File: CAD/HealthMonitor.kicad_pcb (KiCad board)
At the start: 2 copper layers, 70 x 30 mm, 114 parts, among them J1 BAT_T, J10 SDA, J11 SCL, J12 DIS_SW, J13 BAT_CHRG, J14 USBDP, J15 USBDM, J16 USB_V, J17 VBUS, J18 D+, J19 D-, J2 TEG+, J20 SDA, J21 SCL, J22 VCC, J23 GND, J24 BAT_CHRG, J25 DIS_SW, J3 TEG-, J4 BAT-, J5 BAT+, J6 USB_C_Receptacle_USB2.0, J7 Conn_02x05_Odd_Even, J8 VCC, J9 GND, U1 MAX17048G+T10, U10 AT24CS02-XHM, U11 BT832L, U12 CP2102N-A01-GQFN24, U13 ADG884BRMZ, U2 ADP5092ACPZ-1-R7, U3 LTC4079IDD-PBF, U4 LD39015M33R, U5 BH1792GLC, U6 LSM6DS33TR, U7 TXB0104RUT, U8 MAX1921EUT18+, U9 MAX86141ENP+, Y1 ABS06-32.768KHZ-T

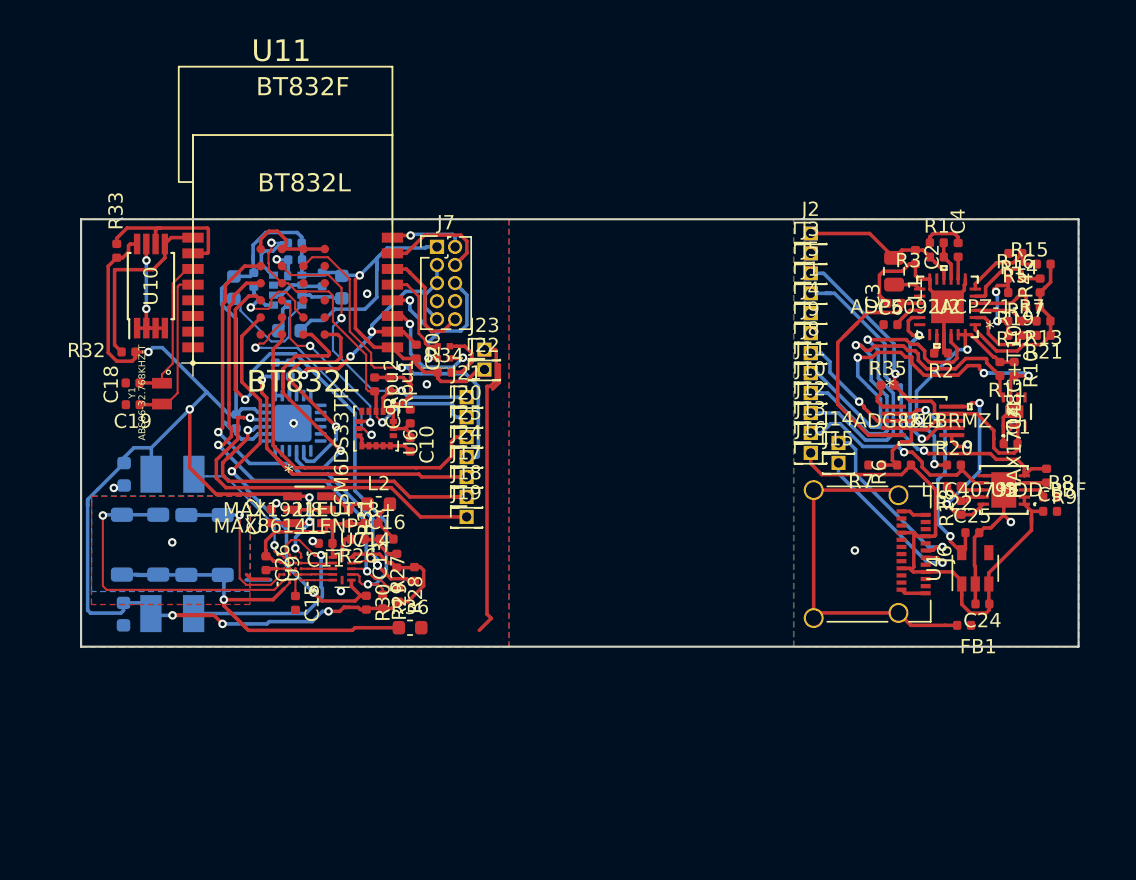
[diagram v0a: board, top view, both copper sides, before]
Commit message: rescue commit
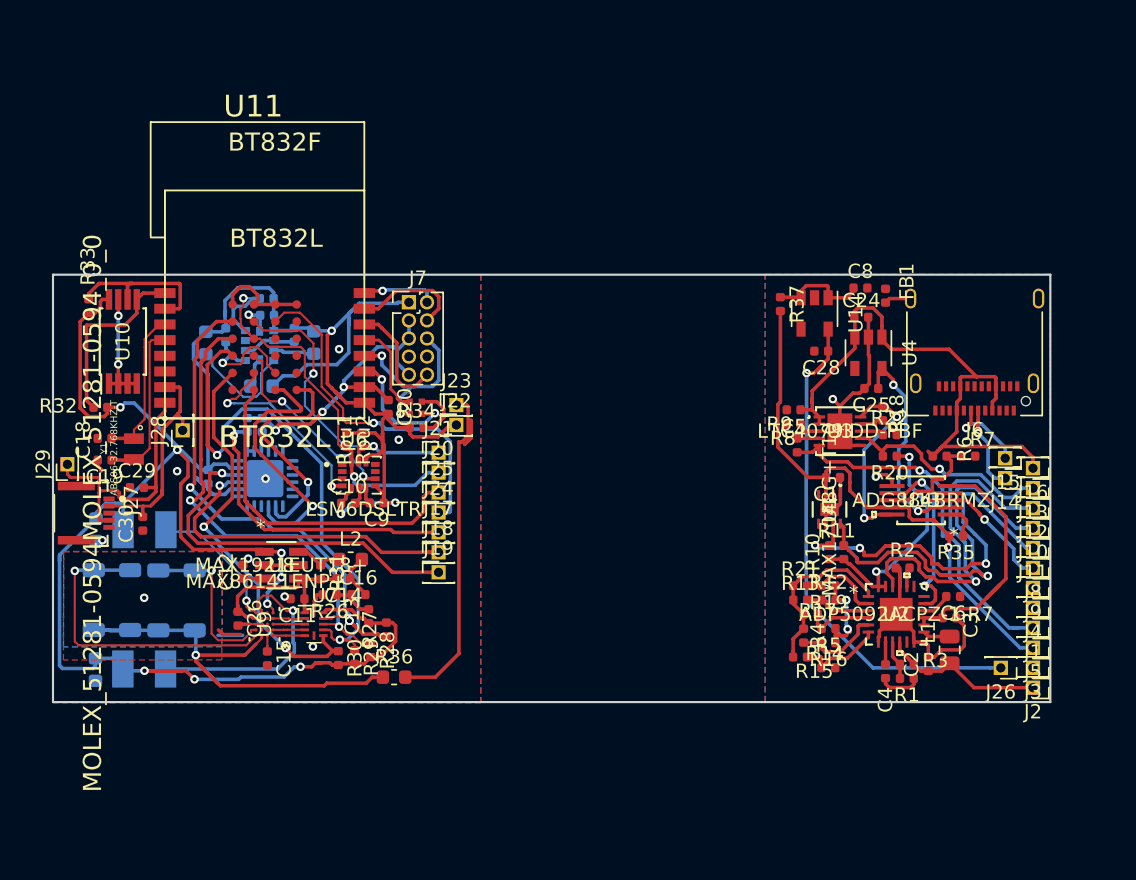
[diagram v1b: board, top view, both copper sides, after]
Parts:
- added C28: 1u, Capacitor_SMD:C_0402_1005Metric, F.Cu at (153.9, 105.4)
- added C29: 12p, Capacitor_SMD:C_0402_1005Metric, F.Cu at (105.9, 114.9)
- added C30: 12p, Capacitor_SMD:C_0402_1005Metric, F.Cu at (106.3, 117.5)
- added C8: 1u, Capacitor_SMD:C_0402_1005Metric, F.Cu at (156.7, 100.9)
- added J26: Conn_01x01_Male, Connector_PinHeader_1.27mm:PinHeader_1x01_P1.27mm_Vertical, F.Cu at (166.5, 127.6)
- added J27: MOLEX_51281-0594MOLEX_51281-0594_0_0, Molex - 51281-0594:Molex - 51281-0594-MOLEX_51281-0594_0, F.Cu at (102.8, 116.7)
- added J28: Conn_01x01_Male, Connector_PinHeader_1.27mm:PinHeader_1x01_P1.27mm_Vertical, F.Cu at (109.1, 110.9)
- added J29: Conn_01x01_Male, Connector_PinHeader_1.27mm:PinHeader_1x01_P1.27mm_Vertical, F.Cu at (101.0, 113.3)
- added R37: 0, Resistor_SMD:R_0402_1005Metric, F.Cu at (151.1, 102.1)
- added U14: LD39015M33R, Package_TO_SOT_SMD:SOT-23-5, F.Cu at (153.4, 102.7)
- C10: value 10µF -> 100nF
- C11, C13: value 0.1µF -> 0.1u
- J6: footprint footprints:USB_C_Receptacle_Amphenol_12401610E4-2A_CircularHoles -> Connector_USB:USB_C_Receptacle_Amphenol_12401610E4-2A
- U6: value LSM6DS33TR -> LSM6DSLTR; footprint LSM6DS33TR:PQFN50P300X300X86-16N -> LSM6DSLTR:PQFN50P300X250X86-14N
- moved J2 35.5 mm to (168.8, 129.0), turned to 180 degrees
- moved J3 33.0 mm to (168.8, 127.6), turned to 180 degrees
- moved R15 32.4 mm to (152.4, 126.8), turned to 0 degrees
- moved R14 31.9 mm to (154.4, 127.6), turned to 180 degrees
- moved R1 30.6 mm to (159.9, 128.3), turned to 180 degrees
- moved J5 30.6 mm to (168.8, 126.2), turned to 180 degrees
- moved C4 30.0 mm to (158.4, 127.8), turned to 270 degrees
- moved R17 29.7 mm to (152.7, 125.3), turned to 270 degrees
- moved R16 28.7 mm to (154.4, 125.8), turned to 180 degrees
- moved R3 28.7 mm to (159.9, 127.3), turned to 0 degrees
- moved C2 28.6 mm to (161.4, 127.3), turned to 90 degrees
- moved J1 28.2 mm to (168.8, 124.8), turned to 180 degrees
- moved R5 27.0 mm to (154.4, 124.8), turned to 180 degrees
- moved L1 26.9 mm to (162.9, 126.3), turned to 270 degrees
- moved R4 26.6 mm to (153.2, 123.8), turned to 180 degrees
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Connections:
- Rpu1 pad 1: +3V3 -> /SCL
- Rpu1 pad 2: /SCL -> +3V3
- U6 pad 1: +3V3 -> GND
- U6 pad 10: GND -> (no net)
- U6 pad 11: GND -> (no net)
- U6 pad 12: GND -> +3V3
- U6 pad 13: GND -> /SCL
- U6 pad 14: Net-(U6-Pad14) -> /SDA
- U6 pad 2: /SCL -> Net-(U6-Pad2)
- U6 pad 3: /SDA -> Net-(U6-Pad3)
- U6 pad 4: /IMUSensor/SDO-SA0 -> /IMU_INT2
- U6 pad 5: /IMUSensor/CS -> +3V3
- U6 pad 6: /IMU_INT1 -> GND
- U6 pad 7: /IMU_INT2 -> GND
- U6 pad 8: GND -> +3V3
- U6 pad 9: GND -> /IMU_INT1
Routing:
- net Net-(C28-Pad1): track 0.00 -> 35.6 mm, vias 0 -> 1
- net Net-(FB1-Pad1): track 25.7 -> 1.88 mm
- net Net-(C29-Pad2): track 0.00 -> 18.7 mm
- net Net-(C30-Pad2): track 0.00 -> 15.5 mm
- net /power/BAT+: track 25.6 -> 39.5 mm
- net +3V3: track 199.6 -> 209.9 mm, vias 13 -> 15
- net Net-(C8-Pad1): track 0.00 -> 7.05 mm
- net /programmer/D+: track 36.4 -> 30.0 mm
- net /programmer/D-: track 37.6 -> 31.3 mm
- net /power/USB_VBUS: track 62.7 -> 65.7 mm
- net GND: track 133.4 -> 131.7 mm
- net /IMU_INT1: track 13.2 -> 14.5 mm
- net Net-(D6-Pad3): track 35.4 -> 36.4 mm
- net /IMU_INT2: track 15.6 -> 14.8 mm
